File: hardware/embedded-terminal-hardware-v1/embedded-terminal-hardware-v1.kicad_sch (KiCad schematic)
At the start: 2 parts, among them J1 USB_C_Receptacle_USB2.0_14P, U1 ATmega328P-A

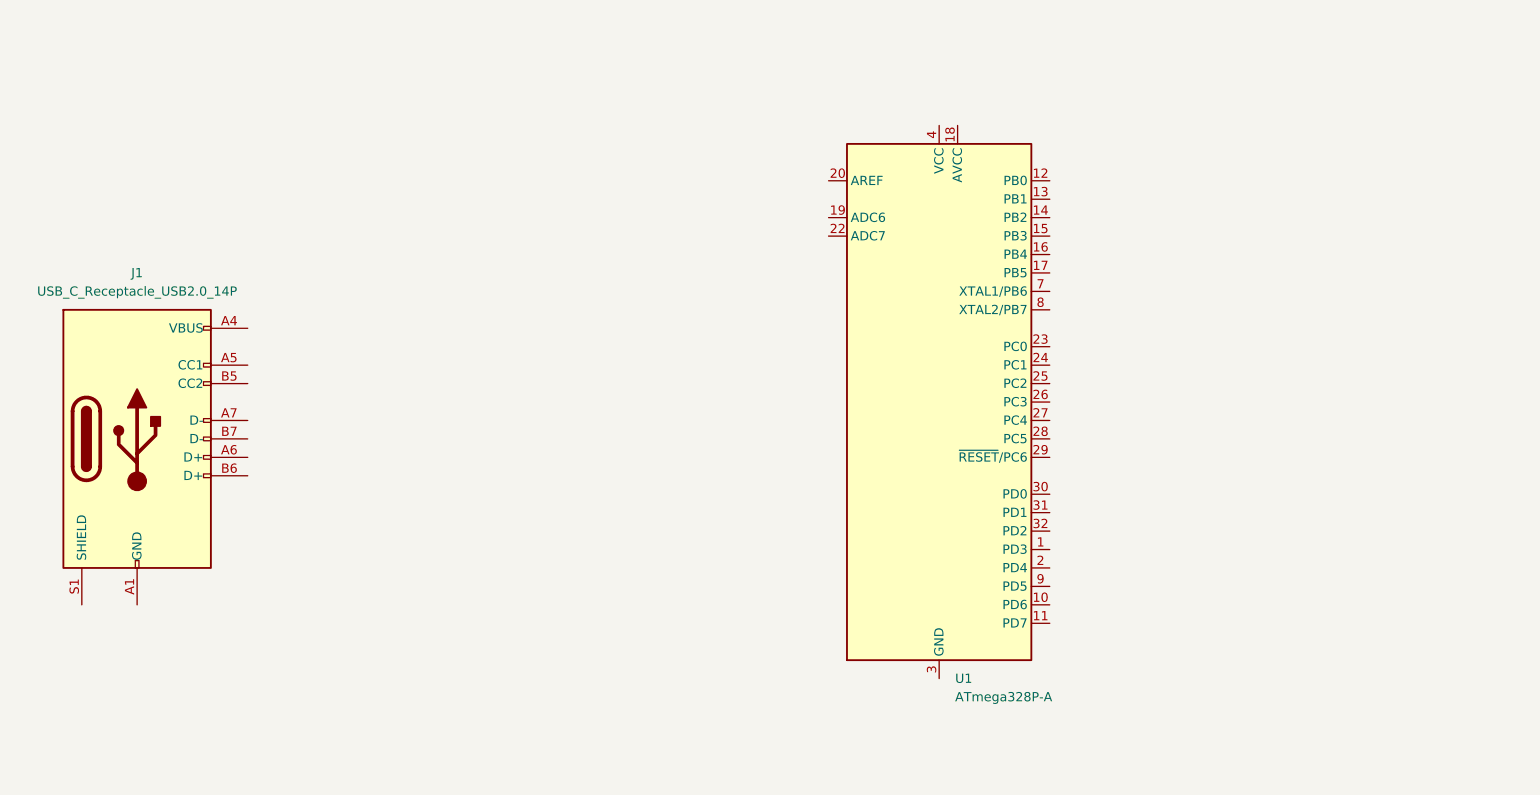
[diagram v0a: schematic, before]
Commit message: Worked on usb
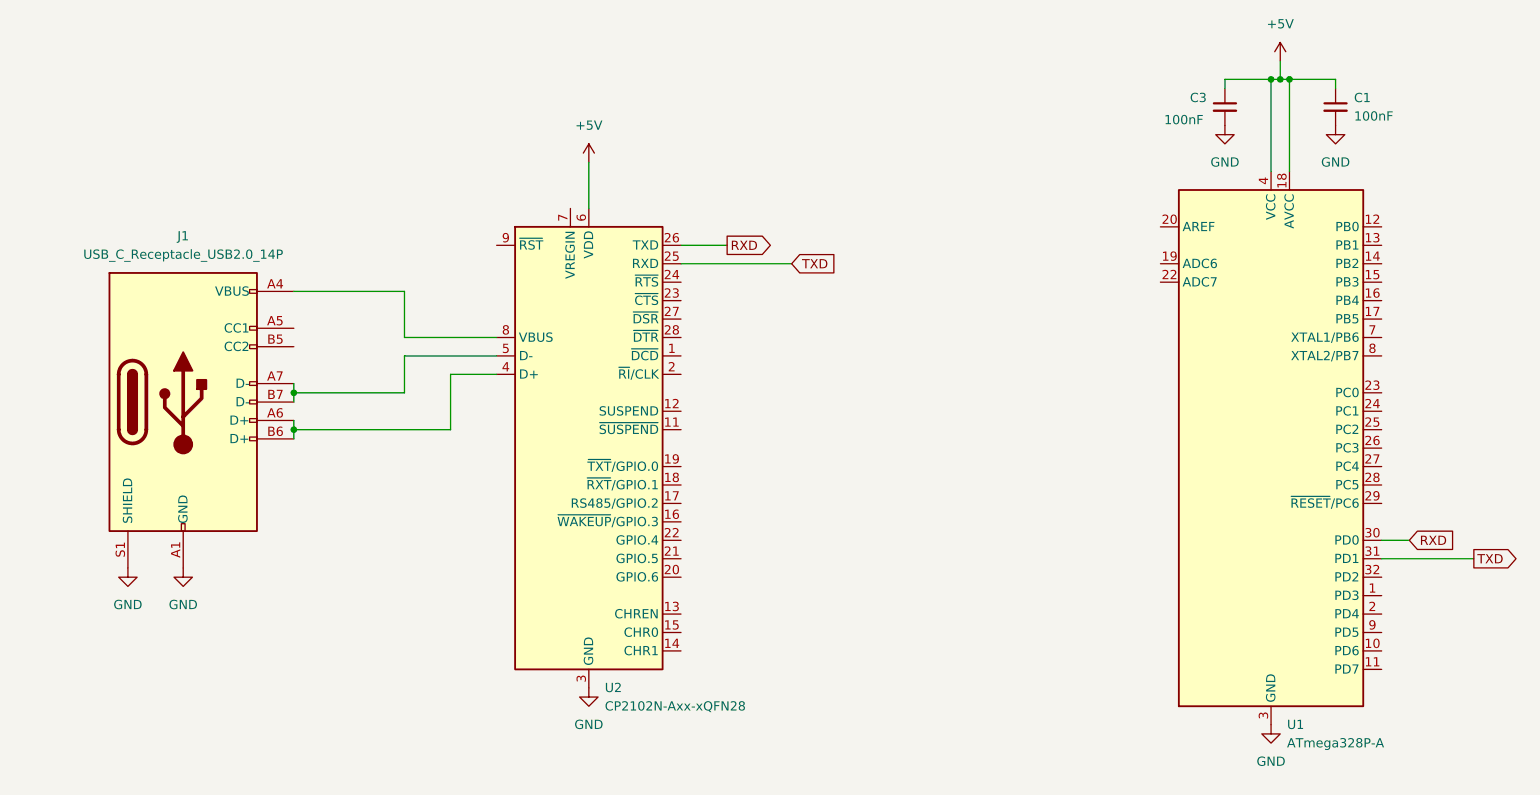
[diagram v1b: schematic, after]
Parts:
- added C1, C3: 100nF, symbol Device:C_Small
- added U2: CP2102N-Axx-xQFN28, Package_DFN_QFN:QFN-28-1EP_5x5mm_P0.5mm_EP3.35x3.35mm, symbol Interface_USB:CP2102N-Axx-xQFN28
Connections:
- net GND: now reaches J1.A1 (GND), J1.A12 (GND), J1.B1 (GND), J1.B12 (GND)
- net GND: now also J1.S1 (SHIELD), U1.21 (GND), U1.3 (GND), U1.5 (GND), C1.2, C3.2, U2.29 (GND), U2.3 (GND)
- net at J1.A4 (VBUS), J1.A9 (VBUS), J1.B4 (VBUS)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: now also U2.8 (VBUS)
- net at J1.A6 (D+): now also J1.B6 (D+), U2.4 (D+)
- net at J1.A7 (D-): now also J1.B7 (D-), U2.5 (D-)
- net +5V: now reaches U1.18 (AVCC)
- net +5V: now also U1.4 (VCC), U1.6 (VCC), C1.1, C3.1, U2.6 (VDD)
- net RXD: now reaches U1.30 (PD0)
- net RXD: now also U2.26 (TXD)
- net TXD: now reaches U1.31 (PD1)
- net TXD: now also U2.25 (RXD)
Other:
- moved on the sheet: J1

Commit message: More work on USB
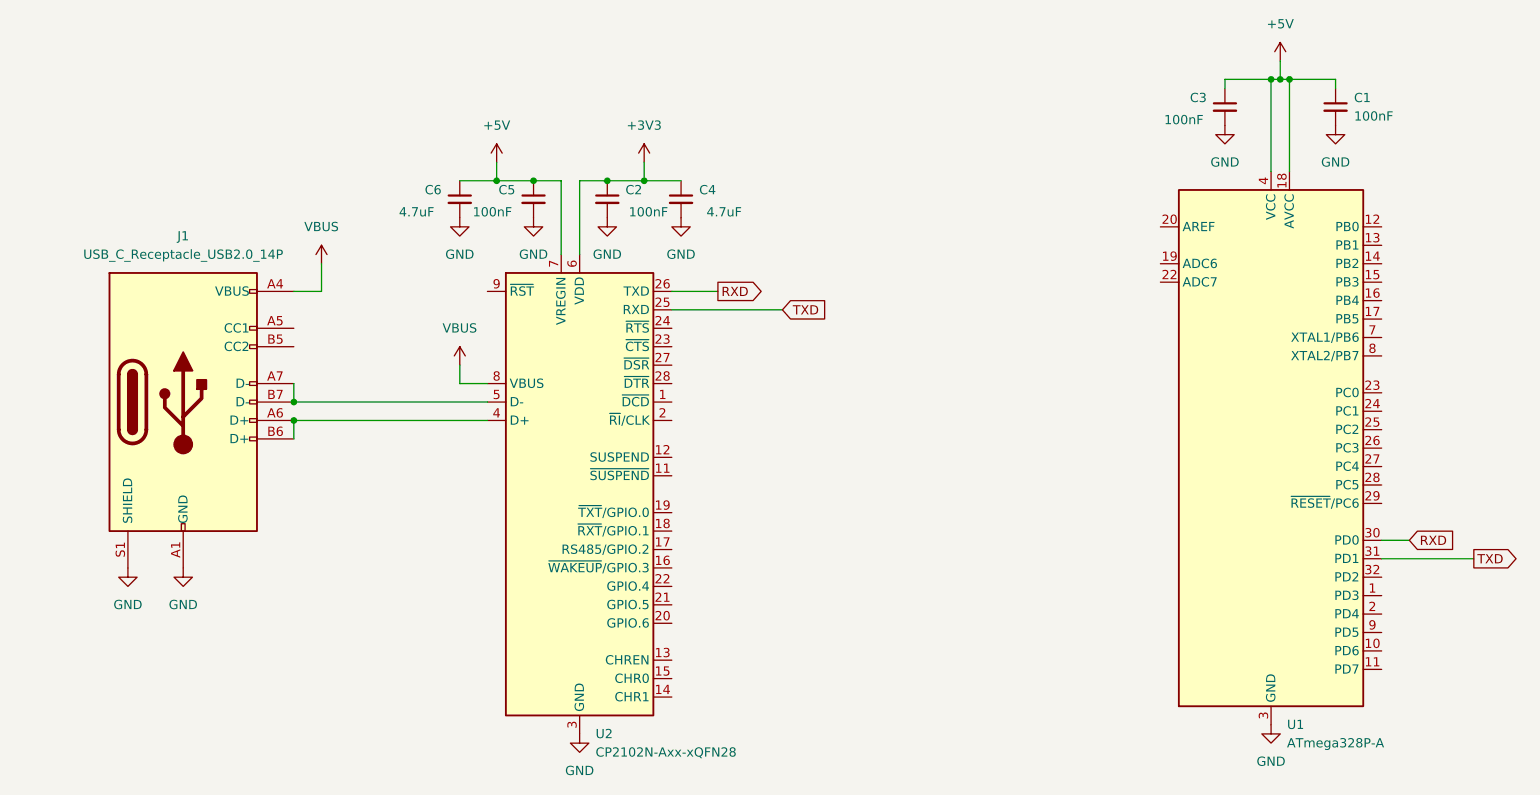
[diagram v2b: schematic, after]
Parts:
- added C2, C5: 100nF, symbol Device:C_Small
- added C4, C6: 4.7uF, symbol Device:C_Small
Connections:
- net +5V: now also U2.7 (VREGIN), C5.1, C6.1; no longer U2.6 (VDD)
- net GND: now also C2.2, C4.2, C5.2, C6.2
- net VBUS: now reaches J1.A4 (VBUS), J1.A9 (VBUS), J1.B4 (VBUS), J1.B9 (VBUS), U2.8 (VBUS)
- new net +3V3: C2.1, C4.1, U2.6 (VDD)
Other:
- moved on the sheet: U2
